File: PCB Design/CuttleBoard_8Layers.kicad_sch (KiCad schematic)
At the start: 170 parts, among them IC1 W25Q256JVEIQ TR, J1 DX07WH24JA3R1200, SW1 SW_Push, SW2 SW_Push, U1 LMR33630CQRNX, U14 STM32H743VIHx, U15 TPS62824ADMQ, U16 ICM-20602, U19 USBLC6-2P6, U20 ACS722xLCTR-10AB, U3 LMR33630CQRNX, U4 ICM-20602, U7 MPRLS0025PA00001A, Y1 NX2016SA

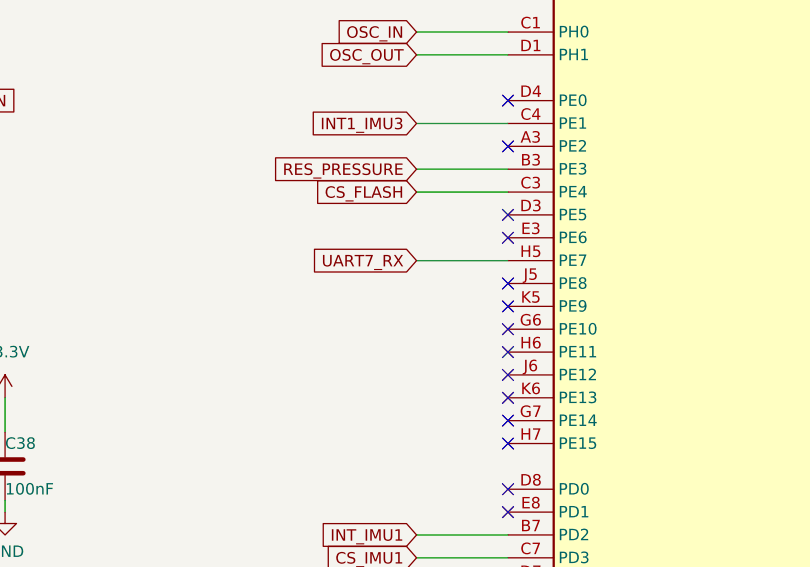
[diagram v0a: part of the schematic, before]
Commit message: fixed errors/warnings, looks OK, needs doublechecking
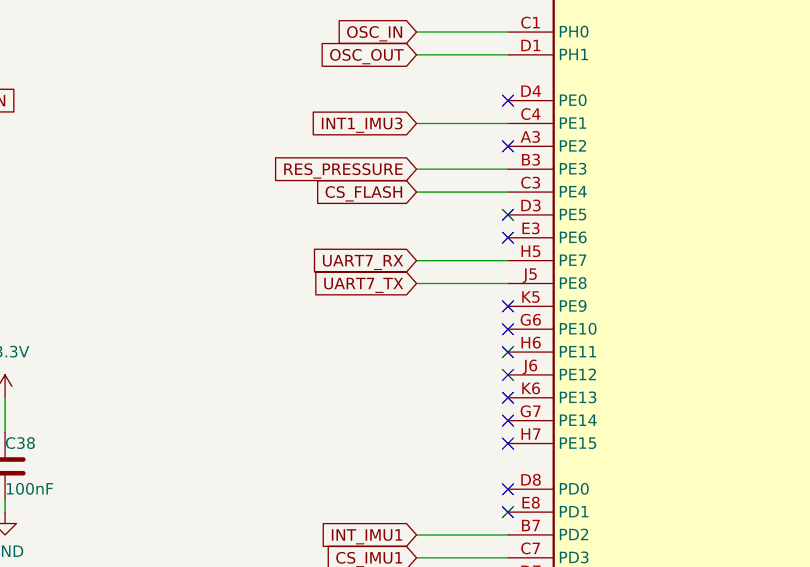
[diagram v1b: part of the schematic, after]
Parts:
- D10, D6, D8, D9: footprint SBRT10U50SP513 -> SBRT10U50SP5:SBRT10U50SP513
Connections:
- net UART7_TX: now also U14.J5 (PE8)
- no-connect marks 69 -> 68
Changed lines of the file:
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@@
 	)
 	(no_connect
-		(at 359.41 81.28)
-	)
-	(no_connect
 		(at 405.13 53.34)
 	)
@@
 	(wire
 		(pts
+			(xy 349.25 81.28) (xy 359.41 81.28)
+		)
+		(stroke
+			(width 0)
+			(type default)
+		)
+	)
+	(wire
+		(pts
 			(xy 368.3 373.38) (xy 341.63 373.38)
 		)
@@
 		)
 	)
+	(global_label "UART7_TX"
+		(shape input)
+		(at 349.25 81.28 180)
+		(effects
+			(font
+				(size 1.27 1.27)
+			)
+			(justify right)
+		)
+		(property "Intersheetrefs" "${INTERSHEET_REFS}"
+			(at 349.25 81.28 0)
+			(effects
+				(font
+					(size 1.27 1.27)
+				)
+				(hide yes)
+			)
+		)
+	)
 	(global_label "I2C3_SDA"
 		(shape input)
@@
 			)
 		)
-		(property "Footprint" "SBRT10U50SP513"
+		(property "Footprint" "SBRT10U50SP5:SBRT10U50SP513"
 			(at 57.15 119.71 0)
 			(effects
@@
 			)
 		)
-		(property "Footprint" "SBRT10U50SP513"
+		(property "Footprint" "SBRT10U50SP5:SBRT10U50SP513"
 			(at 130.48 224.79 0)
 			(effects
@@
 			)
 		)
-		(property "Footprint" "SBRT10U50SP513"
+		(property "Footprint" "SBRT10U50SP5:SBRT10U50SP513"
 			(at 57.15 165.43 0)
 			(effects
@@
 			)
 		)
-		(property "Footprint" "SBRT10U50SP513"
+		(property "Footprint" "SBRT10U50SP5:SBRT10U50SP513"
 			(at 192.71 224.79 0)
 			(effects
